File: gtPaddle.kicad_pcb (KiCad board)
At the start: 2 copper layers, 139.7 x 57.2 mm, 50 parts, among them IC1 74157N, IC2 74157N, J1 Conn_01x02_Pin, J2 Conn_01x02_Pin, J3 Conn_01x02_Pin, J4 Conn_01x02_Pin, Q1 2N3904, Q10 2N3904, Q2 2N3904, Q3 2N3904, Q9 2N3904, U1 ADC0804LCN

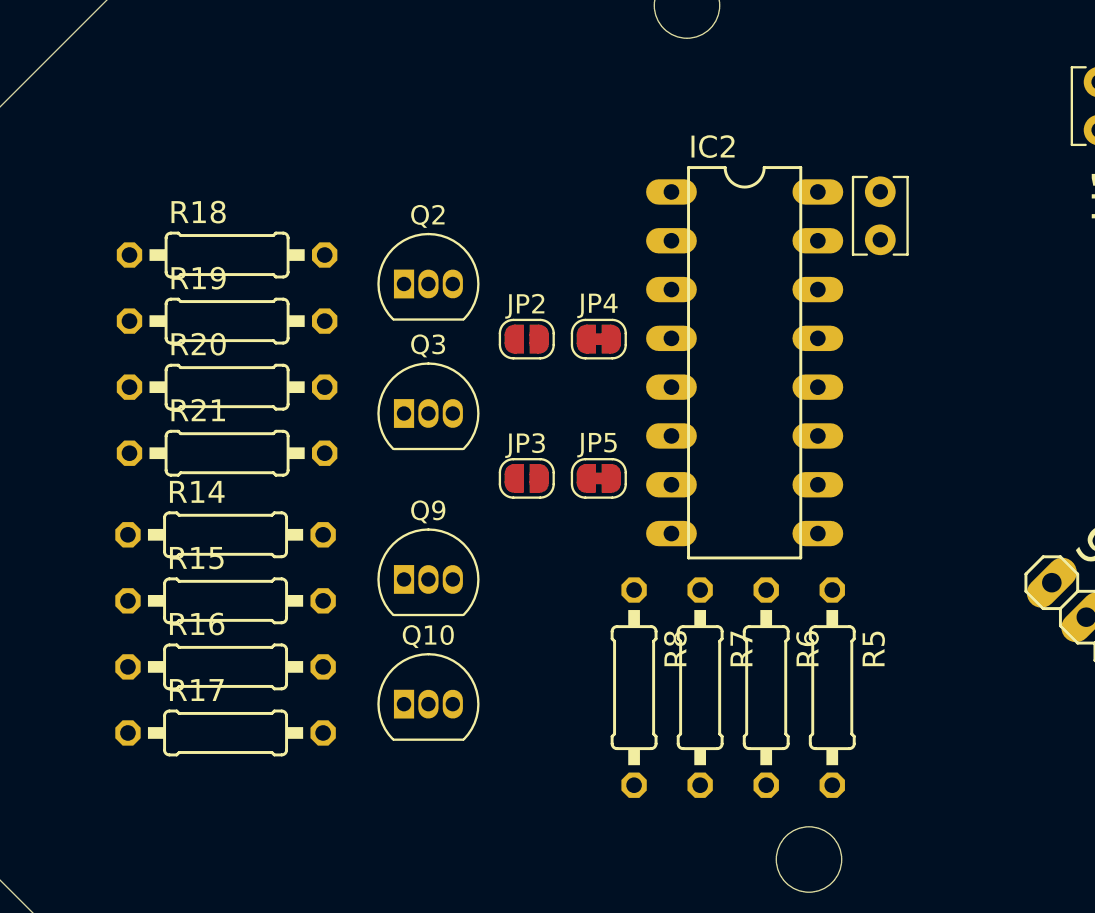
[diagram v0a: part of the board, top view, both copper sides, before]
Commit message: pcb commit before rotating npn mux
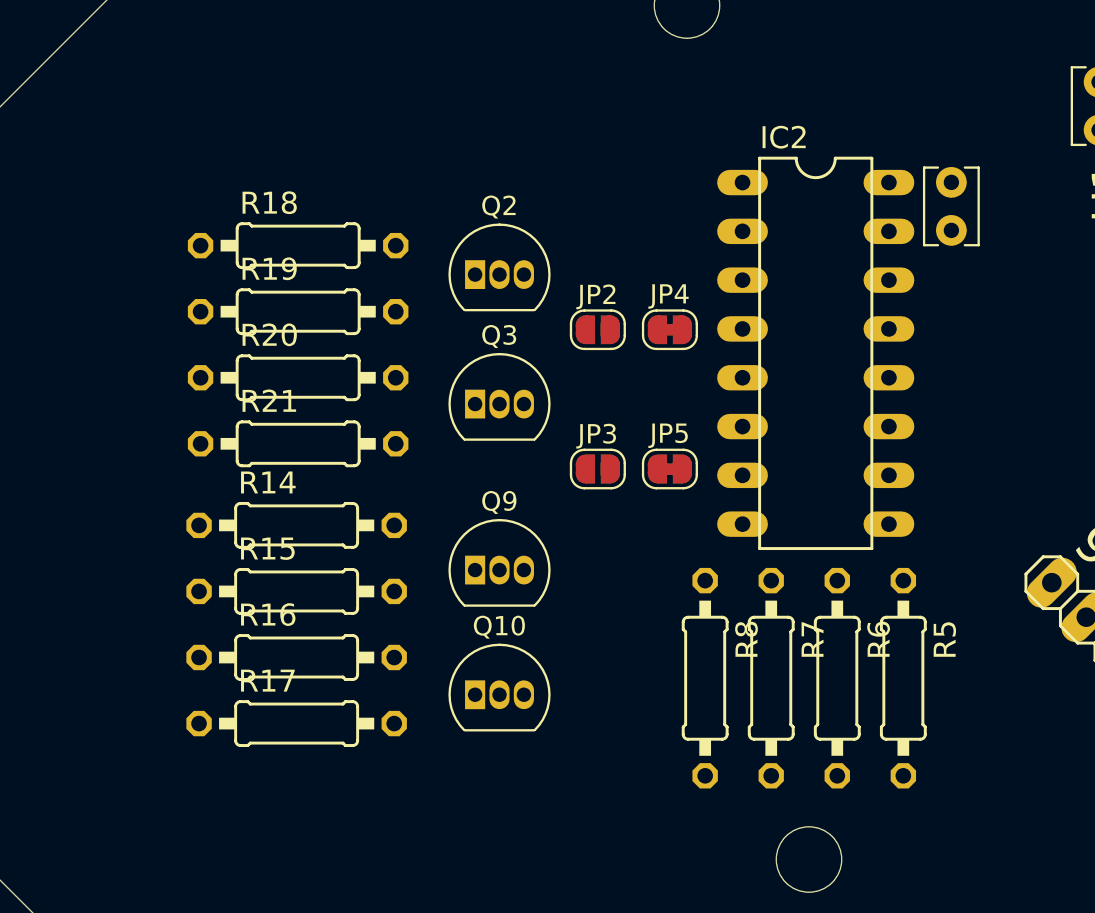
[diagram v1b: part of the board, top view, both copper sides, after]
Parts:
- moved IC2 3.73 mm to (123.6, 91.5)
- moved Q3 3.73 mm to (105.9, 94.1)
- moved Q9 3.73 mm to (105.9, 102.8)
- moved JP2 3.73 mm to (112.3, 90.3)
- moved JP3 3.73 mm to (112.3, 97.5)
- moved JP4 3.73 mm to (116.0, 90.3)
- moved JP5 3.73 mm to (116.0, 97.5)
- moved Q10 3.73 mm to (105.9, 109.3)
- moved Q2 3.73 mm to (105.9, 87.4)
- moved R14 3.73 mm to (96.6, 100.4)
- moved R15 3.73 mm to (96.6, 103.9)
- moved R16 3.73 mm to (96.6, 107.3)
- moved R17 3.73 mm to (96.6, 110.8)
- moved R18 3.73 mm to (96.7, 85.9)
- moved R19 3.73 mm to (96.7, 89.3)
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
